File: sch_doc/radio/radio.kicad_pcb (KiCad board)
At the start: 2 copper layers, 33 parts, among them J1 Conn_01x01, J2 Conn_01x01, J3 Conn_01x01, J4 Conn_01x01, J5 Conn_01x01, J6 Conn_01x01, J8 Conn_01x01, J9 Conn_01x01, Q1 AO3400, U2 TDA7088, U4 LM358

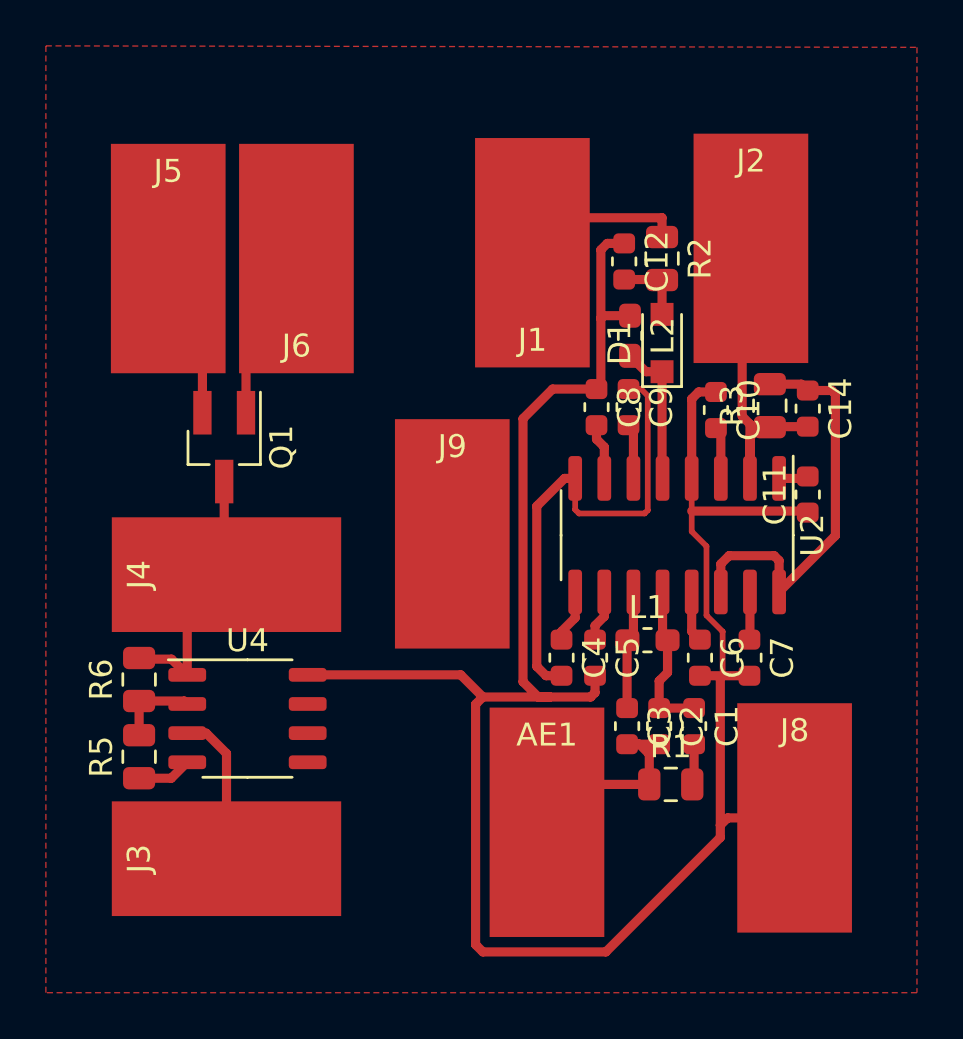
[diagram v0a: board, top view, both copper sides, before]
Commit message: послушал радио с двумя разными усилками и хватит
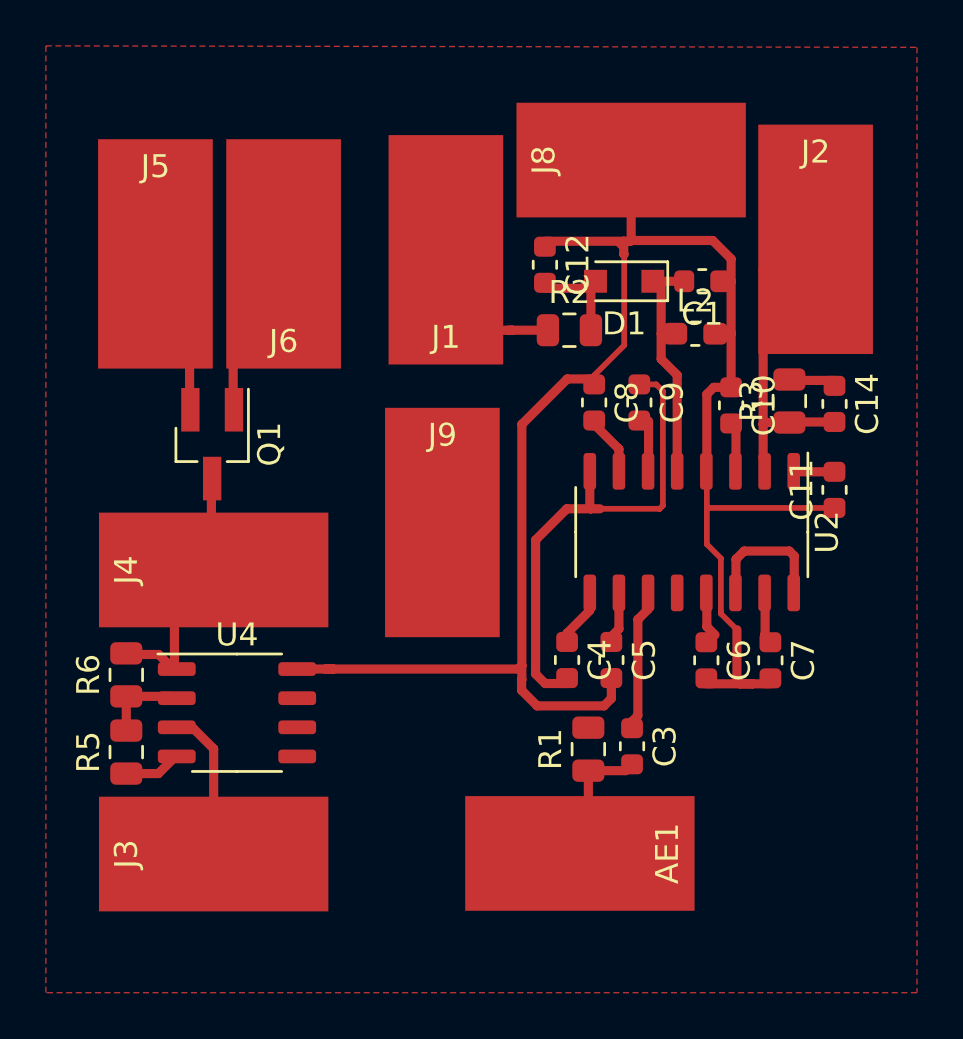
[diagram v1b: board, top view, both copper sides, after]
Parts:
- removed C2: 68pF, Capacitor_SMD:C_0603_1608Metric
- removed L1: 70nH, Inductor_SMD:L_0603_1608Metric_Pad1.05x0.95mm_HandSolder
- C1: value 220pF -> 100pF
- C12: value 680pF -> 330pF
- C3: value 82pF -> 68pF
- D1: value D_Cap -> BB910
- J1: value Conn_01x01 -> tun
- J2, J6: value Conn_01x01 -> out
- J3: value Conn_01x01 -> in_op
- J4: value Conn_01x01 -> in_att
- J5: value Conn_01x01 -> att
- J8: value Conn_01x01 -> vcc
- J9: value Conn_01x01 -> gnd
- L2: value 70nH -> 47nH
- R1: value 3k -> 10k
- U2: footprint Package_SO:SOIC-16_3.9x9.9mm_P1.27mm -> Package_SO:STC_SOP-16_3.9x9.9mm_P1.27mm
- moved J8 29.5 mm to (267.0, 22.3), turned to 90 degrees
- moved C1 19.4 mm to (270.1, 27.5), turned to 180 degrees
- moved R2 5.11 mm to (264.3, 29.7), turned to 0 degrees
- moved R1 3.91 mm to (265.1, 47.9), turned to 90 degrees
- moved J1 3.77 mm to (258.9, 26.2)
- moved C12 3.46 mm to (263.2, 26.8)
- moved D1 3.16 mm to (266.7, 27.5), turned to 180 degrees
- moved J2 2.85 mm to (275.0, 25.7)
- moved L2 2.85 mm to (269.8, 29.8), turned to 0 degrees
- moved AE1 1.98 mm to (264.8, 52.5), turned to 270 degrees
- moved C14 1.19 mm to (275.9, 32.9)
- moved C11 1.19 mm to (275.9, 36.6)
- moved C7 0.92 mm to (273.1, 44.1)
- moved C3 0.90 mm to (267.0, 47.8)
- moved R3 0.87 mm to (273.9, 32.8)
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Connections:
- C1 pad 1: Net-(C1-Pad1) -> +3V3
- D1 pad 1: Net-(D1-Pad1) -> Net-(C1-Pad2)
- L2 pad 1: +3V3 -> Net-(C1-Pad2)
- L2 pad 2: Net-(D1-Pad1) -> +3V3
- R1 pad 2: Net-(C1-Pad2) -> GND
- R5 pad 2: Net-(R5-Pad2) -> GND
- R6 pad 1: Net-(R5-Pad2) -> GND
- U2 pad 12: Net-(C1-Pad1) -> (no net)
- U2 pad 5: Net-(D1-Pad1) -> Net-(C1-Pad2)
- U4 pad 2: Net-(R5-Pad2) -> GND
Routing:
- net +3V3: track 94.3 -> 83.2 mm
- net Net-(C1-Pad2): track 1.79 -> 10.6 mm
- net GND: track 20.4 -> 13.4 mm
- net Net-(C1-Pad1): track 6.83 -> 0.00 mm
- net Net-(D1-Pad1): track 6.34 -> 0.00 mm
- net Net-(C14-Pad2): track 17.9 -> 14.0 mm
- net Net-(AE1-Pad1): track 9.62 -> 5.78 mm
- net Net-(R5-Pad2): track 3.64 -> 0.00 mm
- net Net-(C4-Pad2): track 21.0 -> 23.0 mm
- net Net-(C12-Pad2): track 3.16 -> 4.24 mm
- net Net-(C3-Pad1): track 5.20 -> 5.95 mm
- net Net-(C11-Pad2): track 1.28 -> 1.79 mm
